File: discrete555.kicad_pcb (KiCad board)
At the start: 4 copper layers, 7.6 x 10.2 mm, 44 parts, among them J1 DIP-8, Q1 CET3904E, Q10 CET3906E, Q11 CET3906E, Q12 CET3906E, Q13 CET3906E, Q14 CET3904E, Q15 CET3904E, Q16 CET3904E, Q17 CET3904E, Q18 CET3904E, Q191 CET3906E, Q192 CET3906E, Q2 CET3904E, Q20 CET3904E, Q21 CET3904E, Q22 CET3904E, Q23 CET3906E, Q24 CET3904E, Q25 CET3906E, Q3 CET3904E, Q4 CET3904E, Q5 CET3906E, Q6 CET3906E, Q7 CET3906E, Q8 CET3906E, Q9 CET3906E

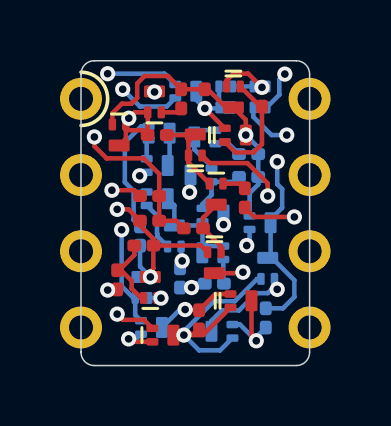
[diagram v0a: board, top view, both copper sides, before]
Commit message: Fussed with top placement a bit more
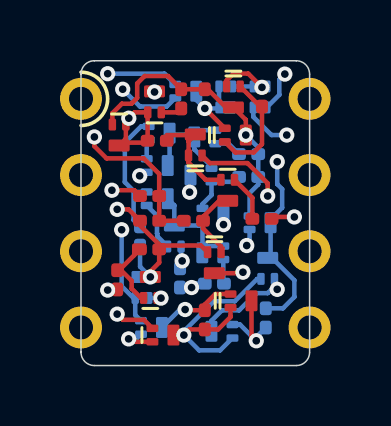
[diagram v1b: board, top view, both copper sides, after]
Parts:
- moved R17 0.90 mm to (44.1, 42.1), turned to 180 degrees
- moved Q25 0.40 mm to (43.0, 41.1)
- moved R16 0.25 mm to (41.8, 42.2)
- moved R9 0.23 mm to (40.4, 43.1)
- moved R10 0.19 mm to (40.6, 39.5)
- moved R6 0.19 mm to (42.2, 45.5)
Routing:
- net ~RST: track 14.2 -> 13.2 mm
- net Net-(Q25-Pad1): track 0.79 -> 1.55 mm
- net Net-(Q14-Pad1): track 1.83 -> 2.53 mm
